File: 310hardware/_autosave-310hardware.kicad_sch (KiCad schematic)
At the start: 10 parts, among them M1 Motor_DC, M2 Motor_DC, M3 Stepper_Motor_bipolar, M4 Stepper_Motor_bipolar, M5 Stepper_Motor_bipolar

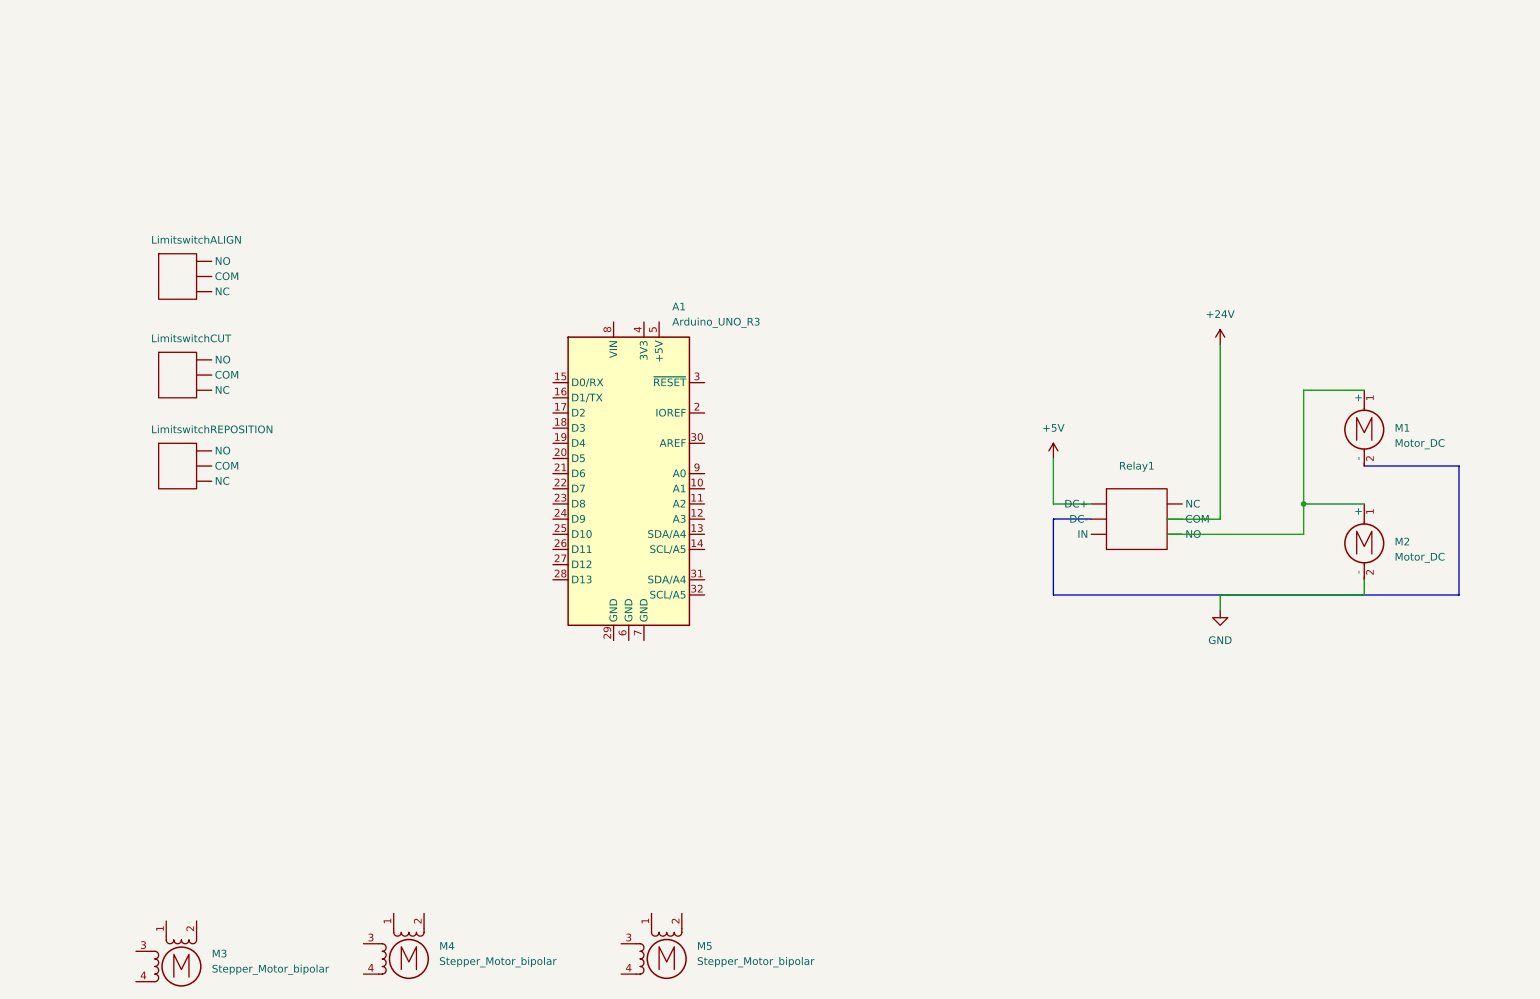
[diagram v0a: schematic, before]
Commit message: Final commit
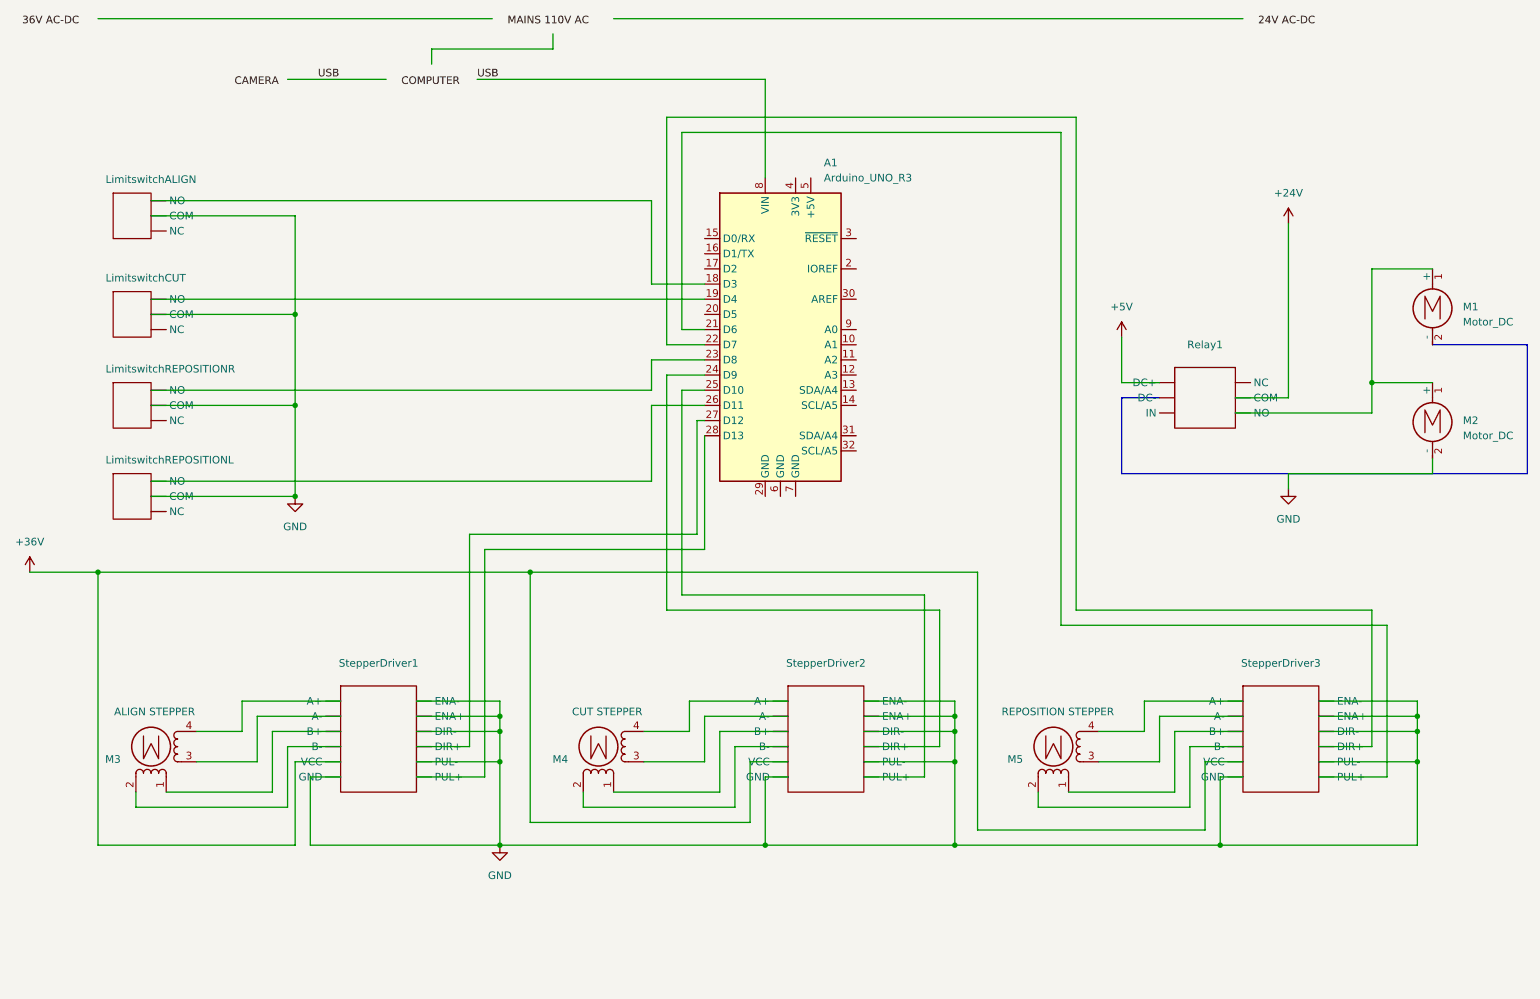
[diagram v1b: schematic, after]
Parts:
- added LimitswitchREPOSITIONL: ~, symbol 310hardwarelib:LImitswitch
- added StepperDriver1, StepperDriver2, StepperDriver3: ~, symbol 310hardwarelib:MicroStepperDriver
- M3: value Stepper_Motor_bipolar -> ALIGN STEPPER
- M4: value Stepper_Motor_bipolar -> CUT STEPPER
- M5: value Stepper_Motor_bipolar -> REPOSITION STEPPER
- renumbered LimitswitchREPOSITION to LimitswitchREPOSITIONR
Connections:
- net GND: now also LimitswitchALIGN. (NO), LimitswitchCUT. (NO), LimitswitchREPOSITIONR. (NO), LimitswitchREPOSITIONL. (NO), StepperDriver1. (VCC), StepperDriver2. (VCC), StepperDriver3. (VCC)
- net at M3.1: now also StepperDriver1. (VCC)
- net at M3.2 (-): now also StepperDriver1. (VCC)
- net at M3.3: now also StepperDriver1. (VCC)
- net at M3.4: now also StepperDriver1. (VCC)
- net at M5.1: now also StepperDriver3. (VCC)
- net at M5.2 (-): now also StepperDriver3. (VCC)
- net at M5.3: now also StepperDriver3. (VCC)
- net at M5.4: now also StepperDriver3. (VCC)
- net at A1.18 (D3): now also LimitswitchALIGN. (NO)
- net at A1.19 (D4): now also LimitswitchCUT. (NO)
- net at A1.21 (D6): now also StepperDriver3. (VCC)
- net at A1.22 (D7): now also StepperDriver3. (VCC)
- net at A1.23 (D8): now also LimitswitchREPOSITIONR. (NO)
- net at A1.24 (D9): now also StepperDriver2. (VCC)
- net at A1.25 (D10): now also StepperDriver2. (VCC)
- net at A1.26 (D11): now also LimitswitchREPOSITIONL. (NO)
- net at A1.27 (D12): now also StepperDriver1. (VCC)
- net at A1.28 (D13): now also StepperDriver1. (VCC)
- net USB: now reaches A1.8 (VIN)
- net at M4.1: now also StepperDriver2. (VCC)
- net at M4.2 (-): now also StepperDriver2. (VCC)
- net at M4.3: now also StepperDriver2. (VCC)
- net at M4.4: now also StepperDriver2. (VCC)
- new net +36V: StepperDriver1. (VCC), StepperDriver2. (VCC), StepperDriver3. (VCC)
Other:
- moved on the sheet: A1, LimitswitchALIGN, LimitswitchCUT, LimitswitchREPOSITIONR, M1, M2, M3, Relay1
